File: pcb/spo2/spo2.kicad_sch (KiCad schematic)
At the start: 14 parts, among them SW1 SW_Push, SW2 SW_Push, SW3 SW_Push, U1 MAX30102, U2 SSD1306

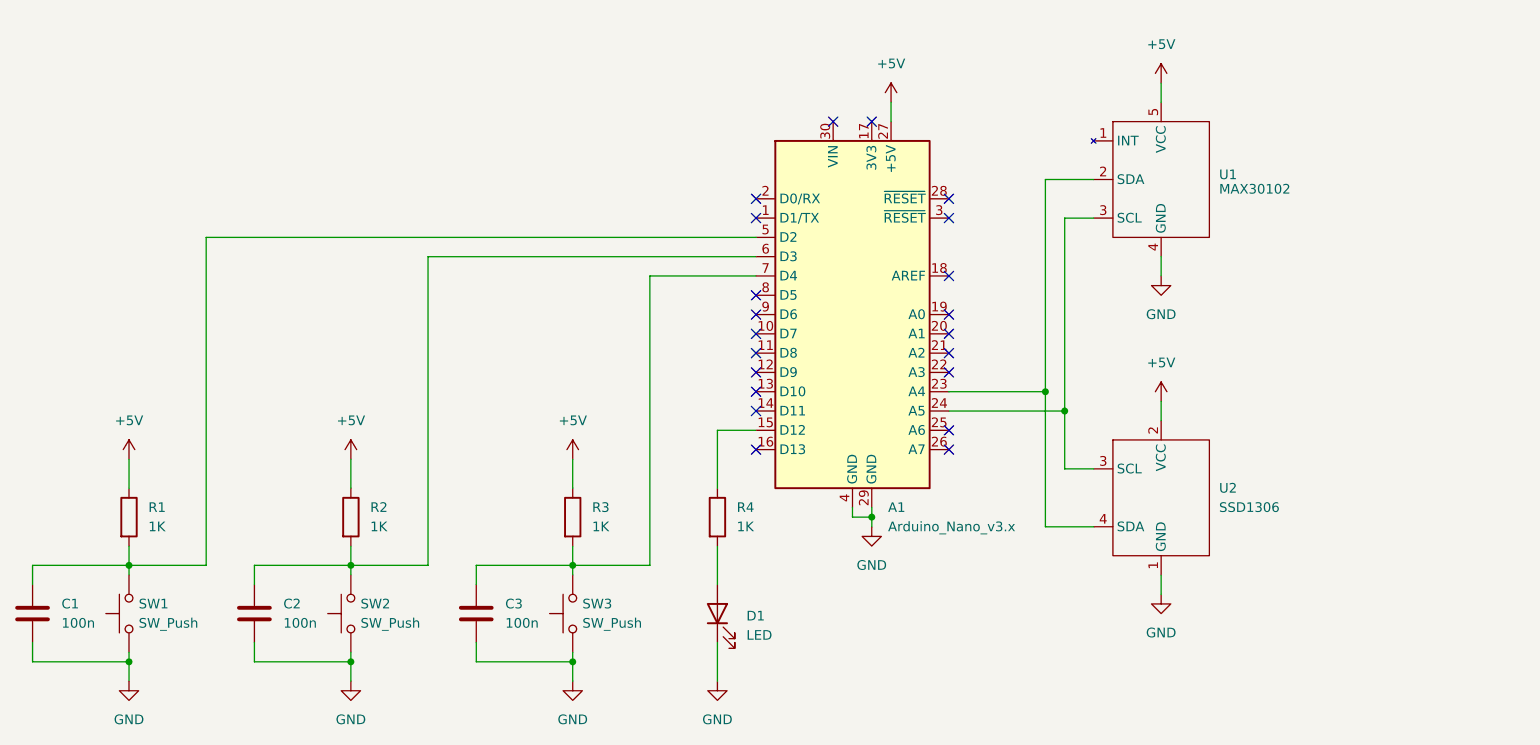
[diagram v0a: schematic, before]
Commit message: Add PCB layout file and Footprint file
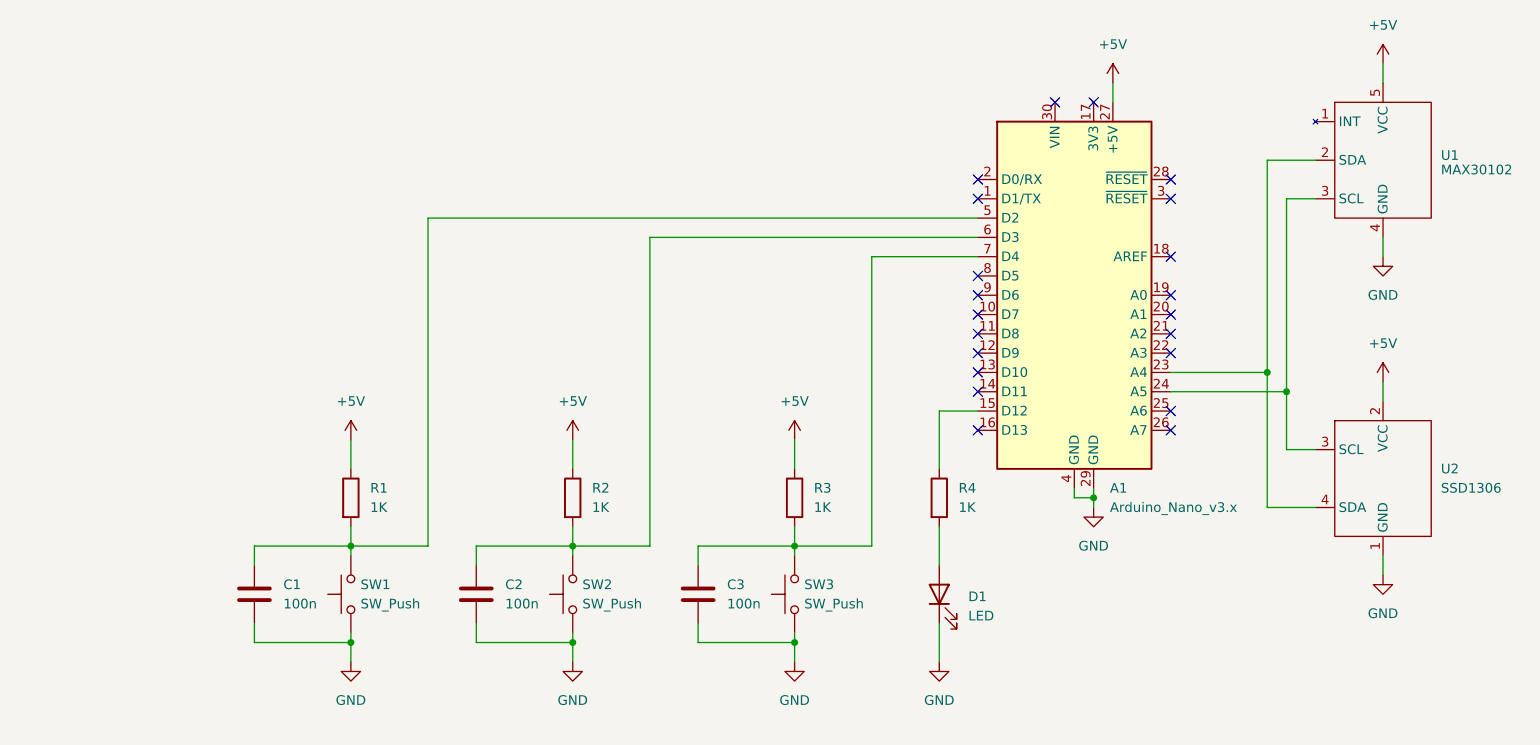
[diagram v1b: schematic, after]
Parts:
- U1: footprint (none) -> spo2_stuff:MAX30102_MODULE
- U2: footprint (none) -> spo2_stuff:SSD1306
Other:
- moved on the sheet: A1, C1, C2, C3, D1, R1, R2, R3, R4, SW1, SW2, SW3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
